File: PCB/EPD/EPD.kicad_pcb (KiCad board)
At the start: 2 copper layers, 28 x 40.5 mm, 63 parts, among them J1 Conn_01x26, J2 Shelly, J3 USB-PROG, J4 BTN1, J6 BTN2, J7 USB-C-Socket-V, J8 PWR, P1 +, P10 2, P11 1, P12 1, P2 -, P3 2, P4 2, P5 1, P6 1, P7 +, P8 -, P9 2, Q1 DMG1012T, U3 MD8942, U4 ESP32-S3-MINI-1

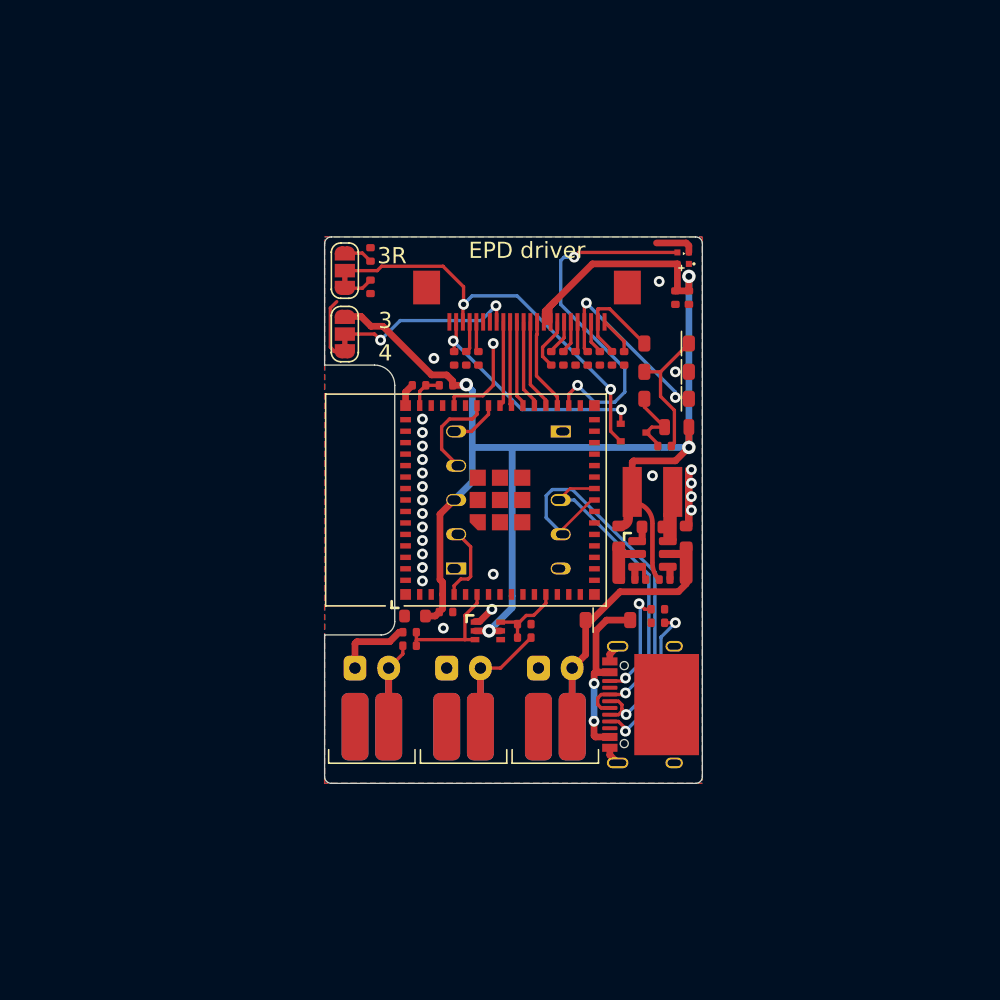
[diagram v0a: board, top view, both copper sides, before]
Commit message: Panel
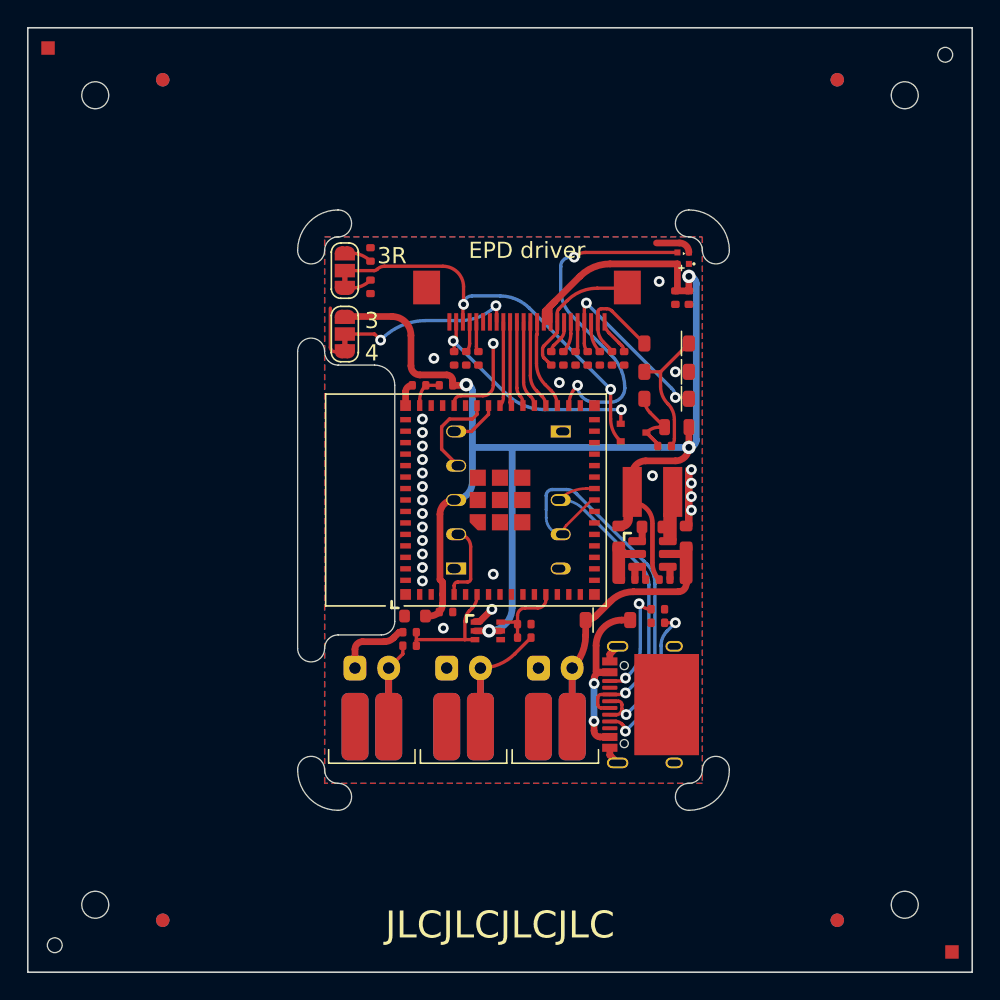
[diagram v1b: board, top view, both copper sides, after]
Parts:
- added PCB1: 70x70, RevK:PCB7070, F.Cu at (99.0, 90.5)
- added V1: ~, RevK:VCUT70N, F.Cu at (114.0, 90.5)
- added V3: ~, RevK:VCUT70N, B.Cu at (86.0, 90.5)
- added V4: ~, RevK:VCUT70N, F.Cu at (99.0, 111.5)
- added V6: ~, RevK:VCUT70N, B.Cu at (99.0, 71.0)
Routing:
- net GND: track 30.4 -> 35.5 mm, vias 25 -> 26
- net Net-(D2-A): track 5.44 -> 6.64 mm
- net +3.3V: track 101.9 -> 102.8 mm
- net Net-(D6-A): track 14.0 -> 13.2 mm
- net Net-(D1-A): track 8.04 -> 7.38 mm
- net D+: track 25.2 -> 24.5 mm
- net Net-(JP2-B): track 2.15 -> 1.60 mm
- net Net-(JP2-A): track 2.15 -> 1.60 mm
- net RGB: track 26.7 -> 26.2 mm
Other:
- board size 28 x 40.5 mm -> 70 x 70 mm
